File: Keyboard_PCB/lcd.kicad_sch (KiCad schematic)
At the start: 11 parts, among them Q2 S8050

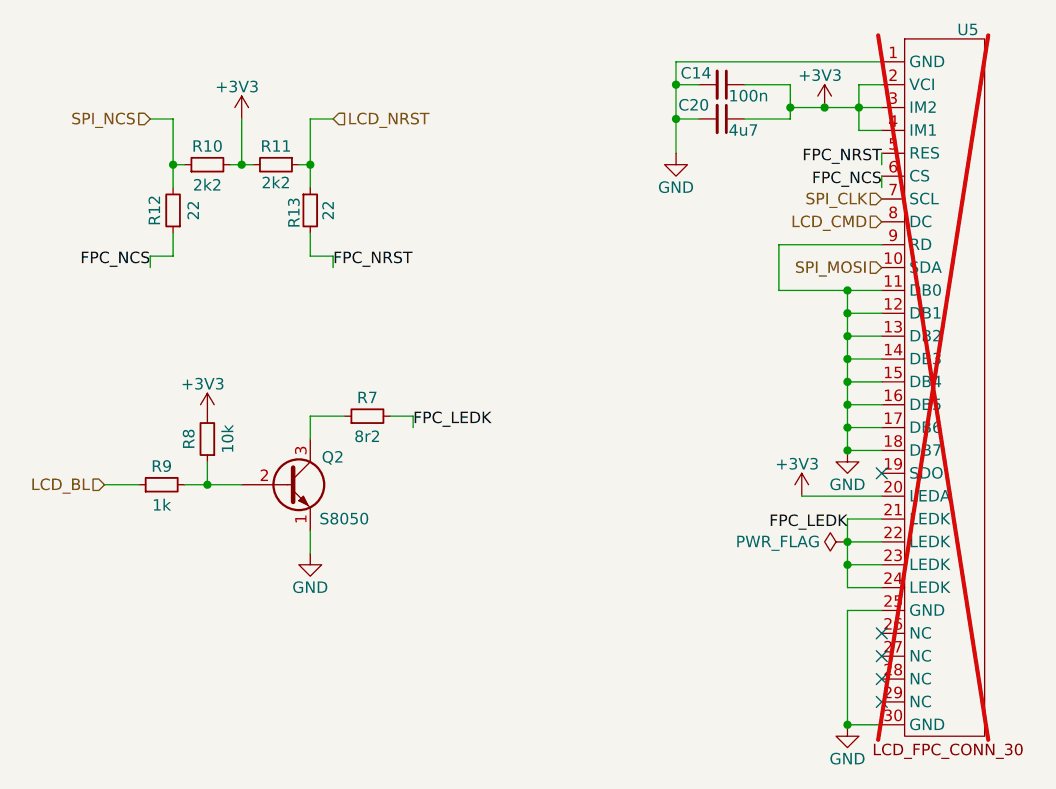
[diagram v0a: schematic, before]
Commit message: Finished Layout V1
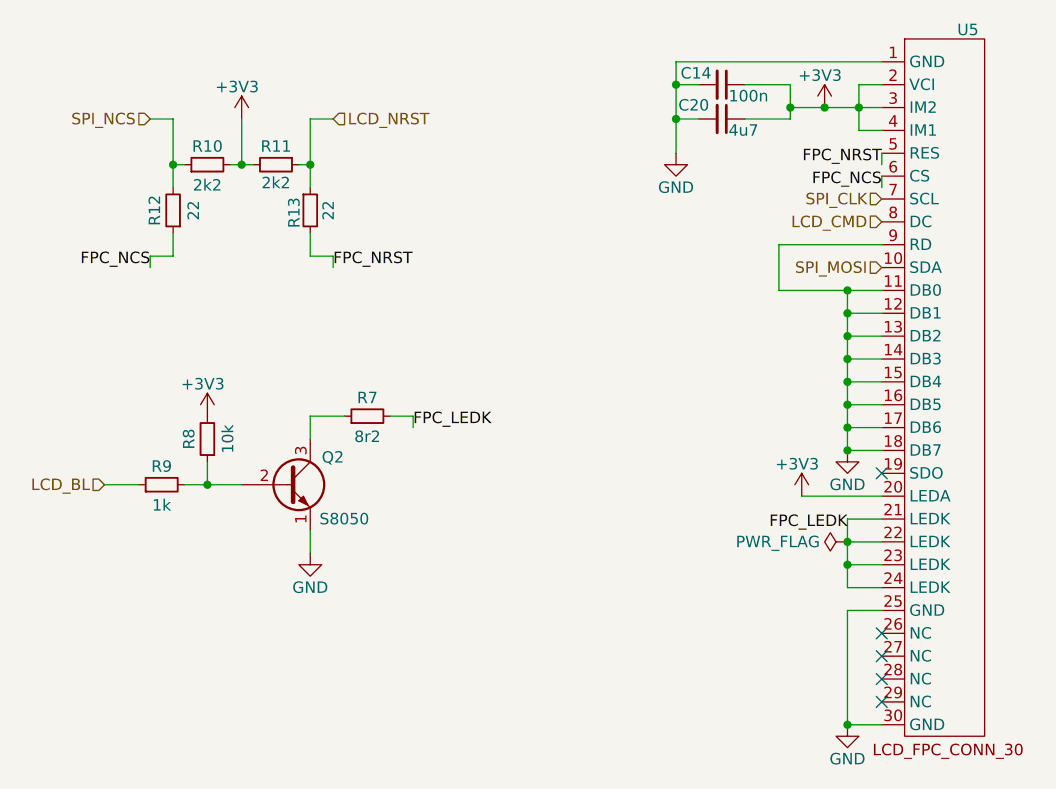
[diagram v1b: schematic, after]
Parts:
- C14: footprint Capacitor_SMD:C_0402_1005Metric -> Capacitor_SMD:C_0603_1608Metric
- C20: footprint Capacitor_SMD:C_0402_1005Metric -> Capacitor_SMD:C_0603_1608Metric; LCSC C23733 -> (none)
- R10, R11, R12, R13, R7, R8, R9: footprint Resistor_SMD:R_0402_1005Metric -> Resistor_SMD:R_0603_1608Metric
- U5: now fitted
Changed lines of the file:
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@@
 			)
 		)
-		(property "Footprint" "Capacitor_SMD:C_0402_1005Metric"
+		(property "Footprint" "Capacitor_SMD:C_0603_1608Metric"
 			(at 191.77 49.53 0)
 			(effects
@@
 			)
 		)
-		(property "LCSC" "C23733"
+		(property "LCSC" ""
 			(at 191.77 49.53 0)
 			(effects
@@
 			)
 		)
-		(property "Footprint" "Resistor_SMD:R_0402_1005Metric"
+		(property "Footprint" "Resistor_SMD:R_0603_1608Metric"
 			(at 129.54 90.17 0)
 			(effects
@@
 			)
 		)
-		(property "Footprint" "Resistor_SMD:R_0402_1005Metric"
+		(property "Footprint" "Resistor_SMD:R_0603_1608Metric"
 			(at 134.62 54.61 0)
 			(effects
@@
 			)
 		)
-		(property "Footprint" "Resistor_SMD:R_0402_1005Metric"
+		(property "Footprint" "Resistor_SMD:R_0603_1608Metric"
 			(at 152.4 82.55 0)
 			(effects
@@
 		(in_bom yes)
 		(on_board yes)
-		(dnp yes)
+		(dnp no)
 		(property "Reference" "U5"
 			(at 217.932 39.624 0)
@@
 			)
 		)
-		(property "Footprint" "Resistor_SMD:R_0402_1005Metric"
+		(property "Footprint" "Resistor_SMD:R_0603_1608Metric"
 			(at 142.24 54.61 0)
 			(effects
@@
 			)
 		)
-		(property "Footprint" "Resistor_SMD:R_0402_1005Metric"
+		(property "Footprint" "Resistor_SMD:R_0603_1608Metric"
 			(at 146.05 59.69 0)
 			(effects
@@
 			)
 		)
-		(property "Footprint" "Capacitor_SMD:C_0402_1005Metric"
+		(property "Footprint" "Capacitor_SMD:C_0603_1608Metric"
 			(at 191.77 45.72 0)
 			(effects
@@
 			)
 		)
-		(property "Footprint" "Resistor_SMD:R_0402_1005Metric"
+		(property "Footprint" "Resistor_SMD:R_0603_1608Metric"
 			(at 134.62 85.09 0)
 			(effects
@@
 			)
 		)
-		(property "Footprint" "Resistor_SMD:R_0402_1005Metric"
+		(property "Footprint" "Resistor_SMD:R_0603_1608Metric"
 			(at 130.81 59.69 0)
 			(effects
